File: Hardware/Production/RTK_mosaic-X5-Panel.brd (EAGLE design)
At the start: 151.8 x 101.6 mm, 408 parts, among them J2 MAGJACK-POE, J3 MICRO-SD-PUSH-PUSH-EXT-PIN, J4 Vertical Qwiic Connector, J9 MAGJACK-POE, T1 TRANSFORMER0508, U1 ESP32-WROVER-IE, U10 POE_PSU-DP990X, U12 URB2405YMD, U2 CH340C, U3 AP7361C-33FGEUDFN-8, U6 AP7361C-33FGEUDFN-8, U7 KSZ8041NLI, U8 MOSAIC-X5X5, U9 KSZ8041NLI

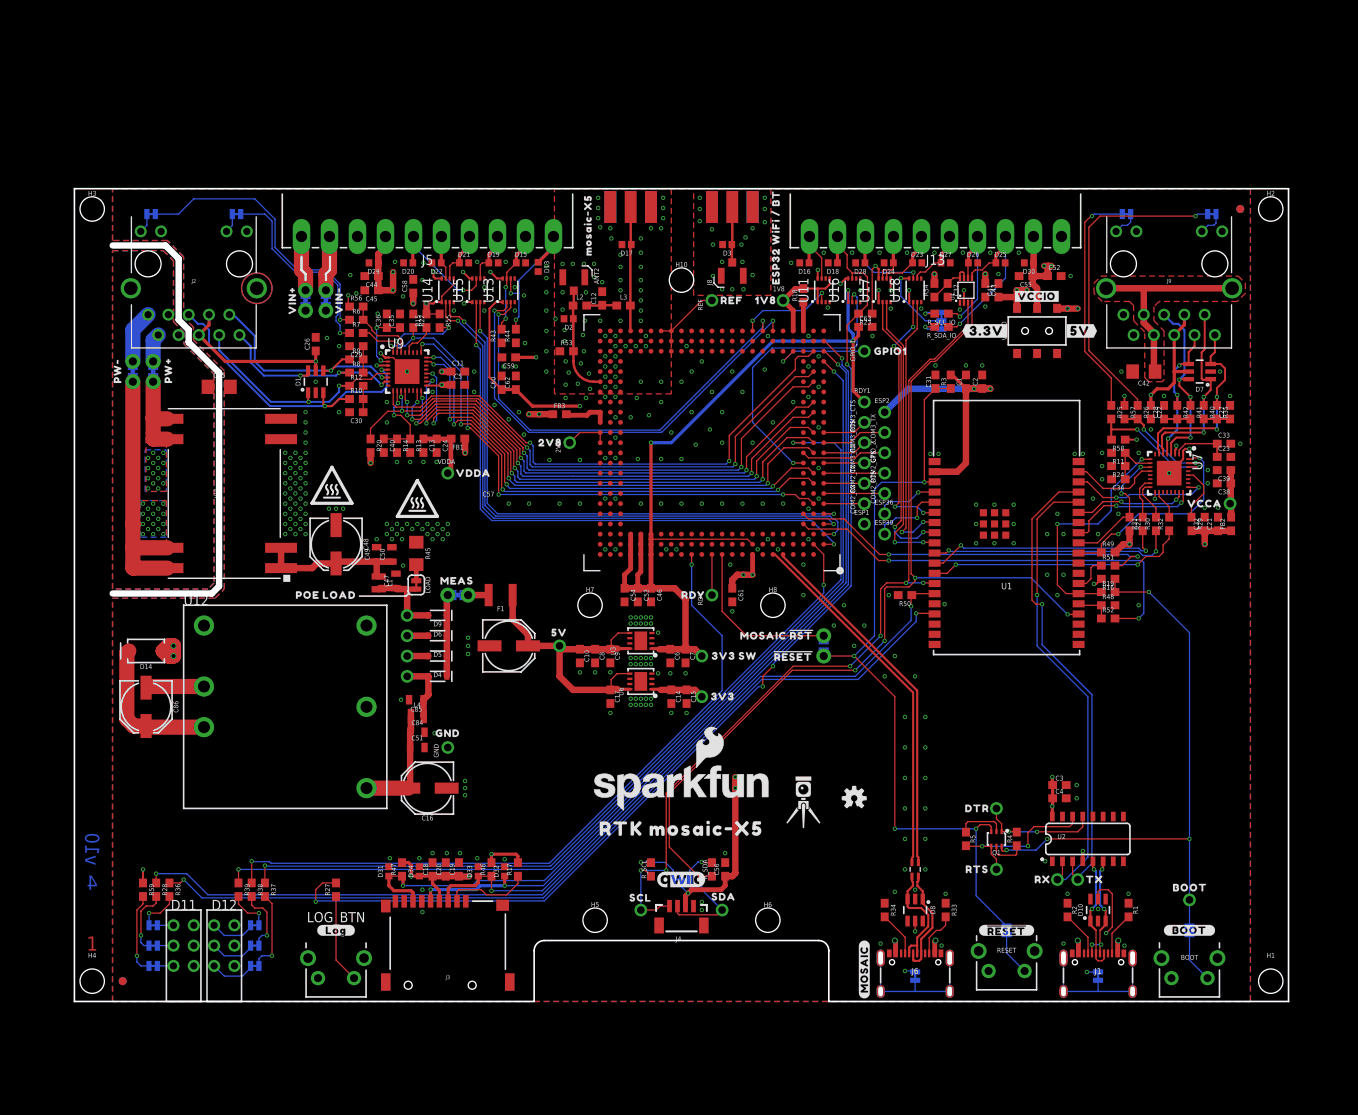
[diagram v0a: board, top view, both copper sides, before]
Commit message: v10 - ready for manufacture
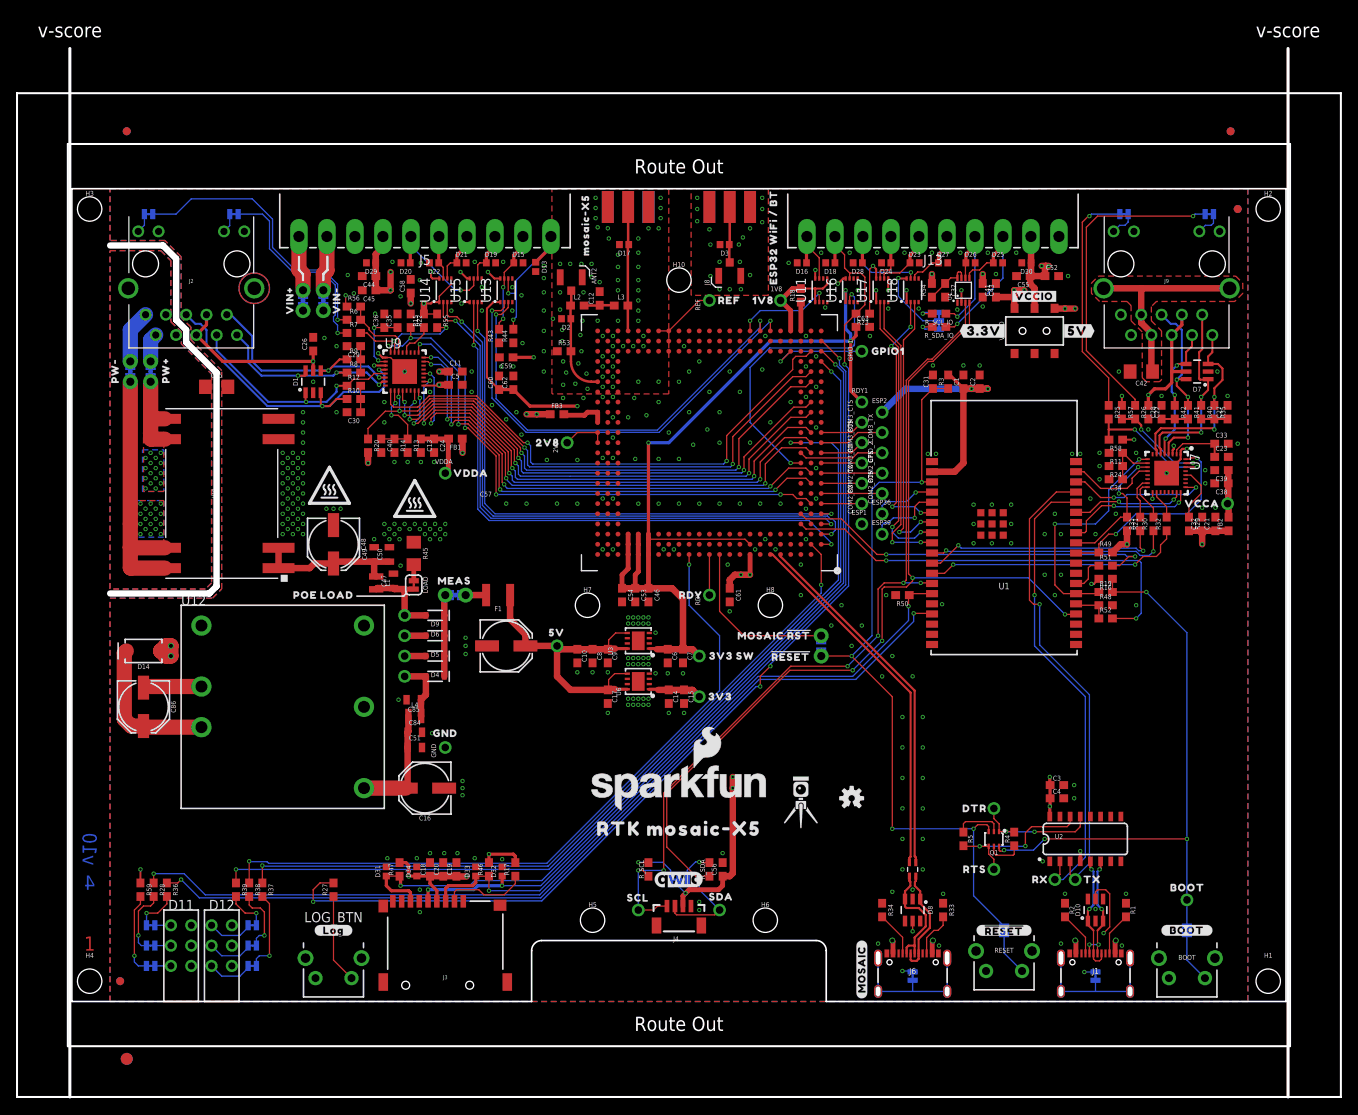
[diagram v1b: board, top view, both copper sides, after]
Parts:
- removed FRAME1: FRAME-LEDGER, SparkFun-Aesthetics:CREATIVE_COMMONS
- removed FRAME3: FRAME-LEDGERNO_FOOTPRINT, SparkFun-Aesthetics:DUMMY
- removed LOGO1: SPECIAL_INSTRUCTIONS-ORDERING, SparkFun-Aesthetics:ORDERING_INSTRUCTIONS
- added E$1, E$2, E$3, E$4: (no value), SparkFun-Aesthetics:FIDUCIAL-1X2
- added E$5, E$6: (no value), SparkFun-Retired:FIDUCIAL-1.5X3
- moved FB2 0.32 mm to (144.6, 59.7)
- moved FD3 0.32 mm to (145.7, 99.1)
- moved FD4 0.32 mm to (145.7, 99.1)
- moved H1 0.32 mm to (149.5, 2.54)
- moved H2 0.32 mm to (149.5, 99.1)
- moved R1 0.32 mm to (131.8, 11.4)
- moved R26 0.32 mm to (132.9, 73.7)
- moved 1V8 0.32 mm to (88.6, 87.6)
- moved C1 0.32 mm to (111.4, 77.5)
- moved C14 0.32 mm to (74.6, 38.1)
- moved C3 0.32 mm to (123.1, 27.1)
- moved C31 0.32 mm to (107.6, 77.5)
- moved C37 0.32 mm to (109.2, 88.9)
- moved C4 0.32 mm to (123.1, 25.4)
- moved C53 0.32 mm to (70.4, 50.8)
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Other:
- board size 151.8 x 101.6 mm -> 165.5 x 131.1 mm
- board text added: "Route Out"
- board text added: "v-score"
- board text removed: "Controlled Impedance: JLC7628 Material: TG155 4-Layers Thickness: 1.6mm Outer Copper: 1oz Inner Copper: 0.5oz Finish: ENIG Red Solder Resist White Silkscreen No clean process"
- board text removed: "Dimensions In Inches"
- board text removed: "Paul Clark"
- board text removed: "V-Score To V-Score"
